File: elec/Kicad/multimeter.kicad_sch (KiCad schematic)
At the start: 6 parts, among them J3 HX0201800000G

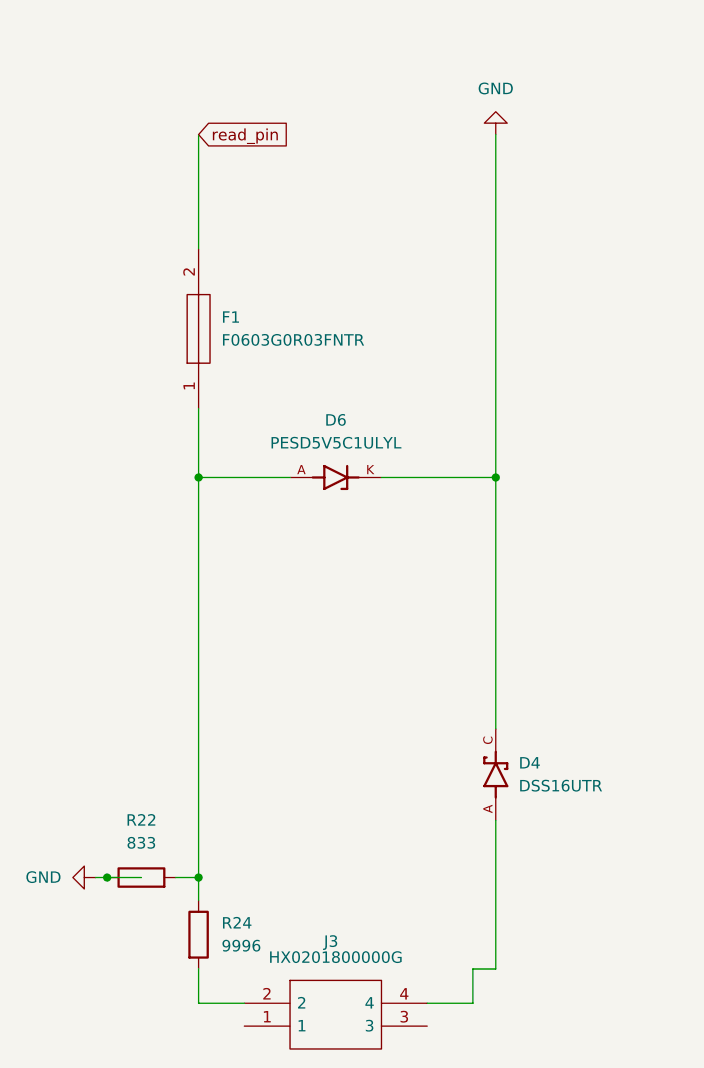
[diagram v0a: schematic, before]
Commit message: multimetre final
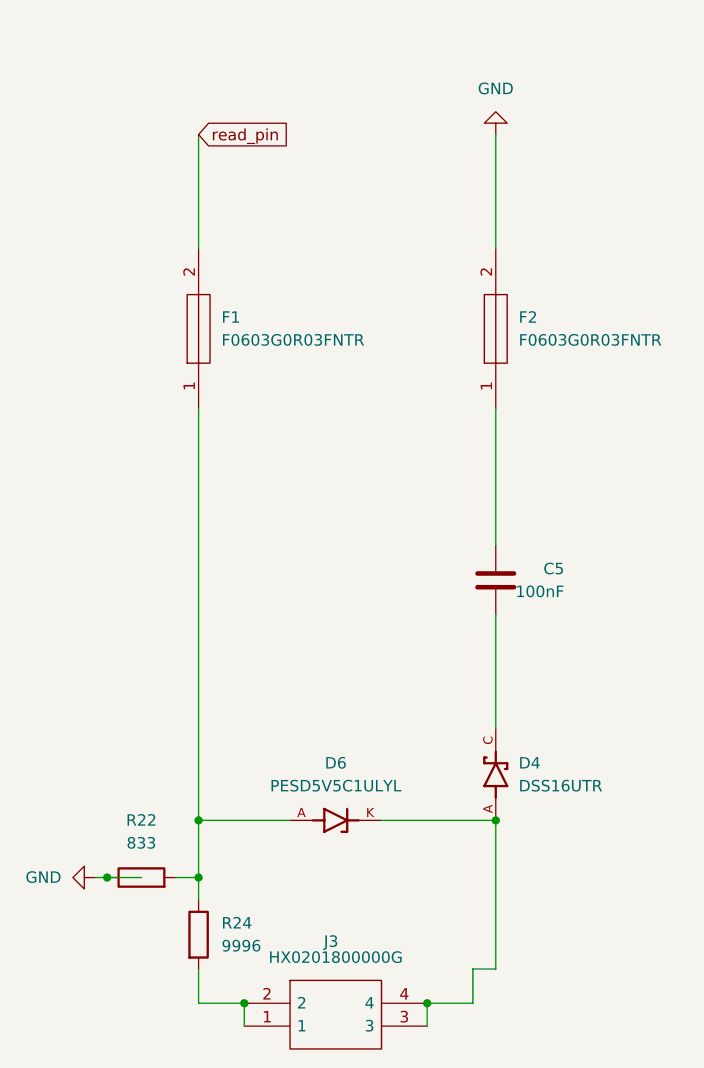
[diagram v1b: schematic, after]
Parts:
- added C5: 100nF, Capacitor_SMD:C_0603_1608Metric_Pad1.08x0.95mm_HandSolder, symbol Device:C
- added F2: F0603G0R03FNTR, F0603G0R03FNTR:F0603G0R03FNTR, symbol F0603G0R03FNTR:F0603G0R03FNTR
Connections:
- net GND: now also F2.2; no longer D4.C, D6.K
- net at J3.1: now also J3.2, R24.2
- net at J3.3: now also D4.A, D6.K, J3.4
- new net: C5.1, F2.1
- new net: C5.2, D4.C
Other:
- moved on the sheet: D6

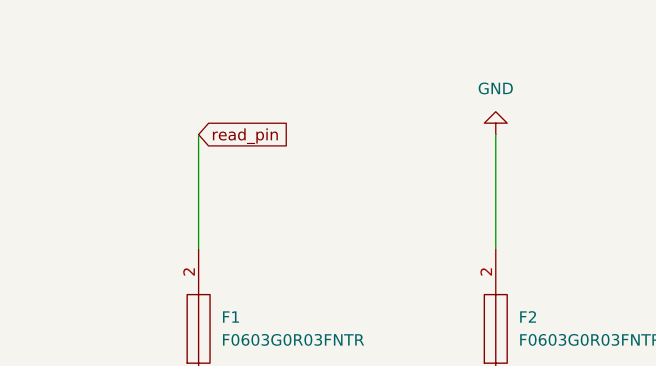
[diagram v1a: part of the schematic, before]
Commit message: touillerie
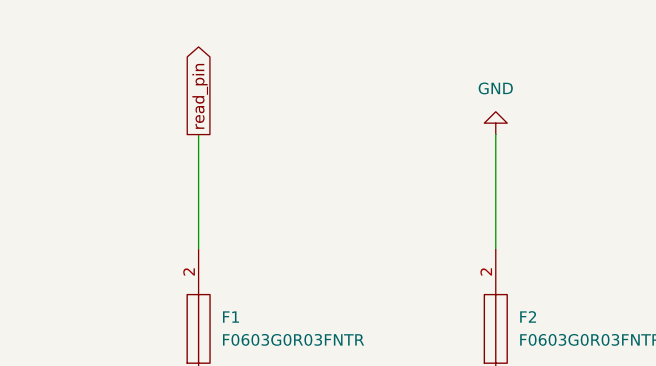
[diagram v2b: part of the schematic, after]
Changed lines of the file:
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@@
 	)
 	(global_label "read_pin"
-		(shape input)
-		(at 36.83 29.21 0)
+		(shape output)
+		(at 36.83 29.21 90)
 		(fields_autoplaced yes)
 		(effects
@@
 		)
 		(property "Intersheetrefs" "${INTERSHEET_REFS}"
-			(at 47.8584 29.21 0)
+			(at 36.83 18.1816 90)
 			(effects
 				(font
